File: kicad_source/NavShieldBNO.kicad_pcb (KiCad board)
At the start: 2 copper layers, 36 x 23 mm, 40 parts, among them CN1 ARDUINO_MKR, CN2 CONN_01X04, CN3 CONN_01X04, U1 BNO085, U2 BMP388

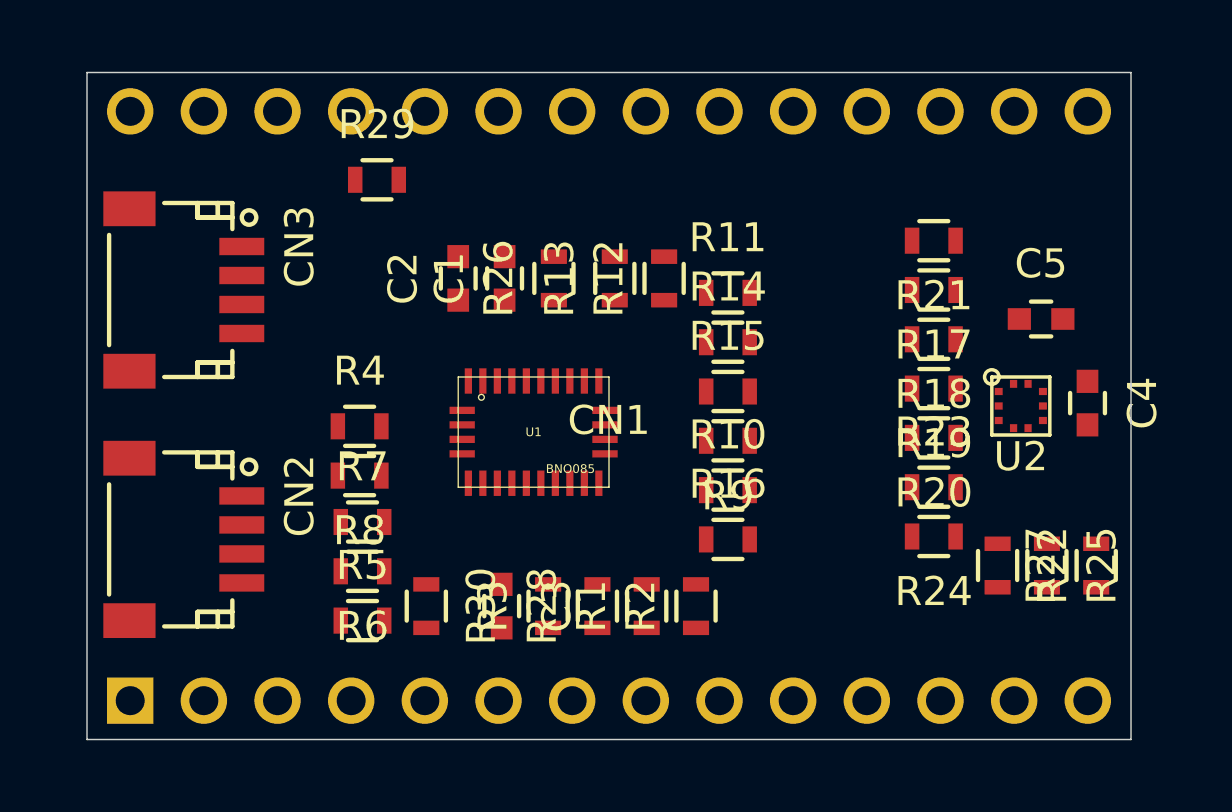
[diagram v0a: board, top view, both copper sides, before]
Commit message: first draft of layout
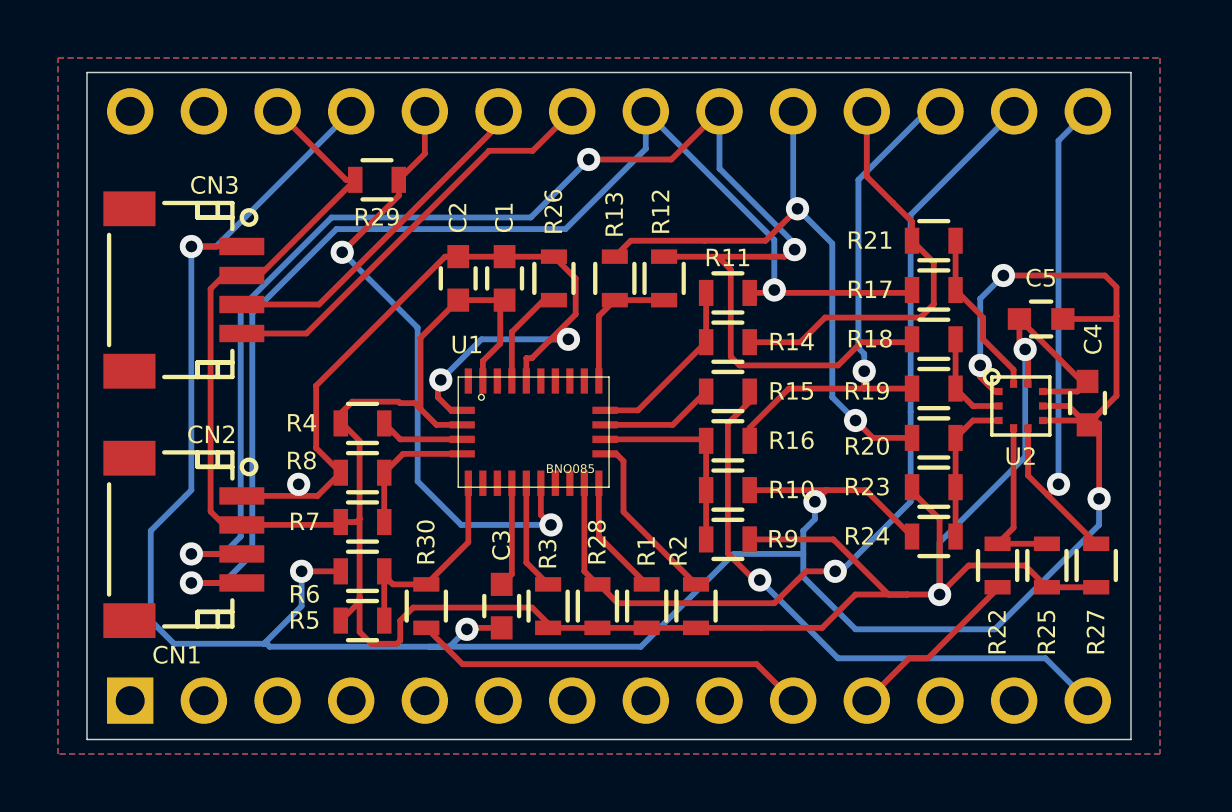
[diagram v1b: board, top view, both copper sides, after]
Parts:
- moved R16 3.40 mm to (107.1, 161.2)
- moved R9 3.40 mm to (107.1, 164.6)
- moved R4 0.14 mm to (94.5, 160.6)
- moved R8 0.14 mm to (94.5, 162.3)
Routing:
- net GND: track 0.00 -> 129.0 mm, vias 0 -> 10
- net +3V3: track 0.00 -> 101.2 mm, vias 0 -> 2
- net /I2C_SDA: track 0.00 -> 51.7 mm, vias 0 -> 3
- net /I2C_SCL: track 0.00 -> 43.5 mm, vias 0 -> 2
- net /BNO085_INT: track 0.00 -> 31.1 mm, vias 0 -> 1
- net /RESET: track 0.00 -> 21.8 mm, vias 0 -> 2
- net /SPI_MISO: track 0.00 -> 20.7 mm, vias 0 -> 2
- net /BNO085_CS: track 0.00 -> 20.4 mm, vias 0 -> 1
- net /BMP388_INT: track 0.00 -> 18.8 mm, vias 0 -> 1
- net /SPI_MOSI: track 0.00 -> 17.7 mm, vias 0 -> 1
- net /SERIAL_RX: track 0.00 -> 14.6 mm
- net /SPI_SCK: track 0.00 -> 14.5 mm
- net /WAKE: track 0.00 -> 13.7 mm
- net /SERIAL_TX: track 0.00 -> 11.9 mm
- net /PS0: track 0.00 -> 7.51 mm
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- added copper zone on B.Cu, net GND
- added copper zone on F.Cu, net GND
